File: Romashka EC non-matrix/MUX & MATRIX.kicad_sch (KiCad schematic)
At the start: 65 parts, among them SW1 EC_SW, SW10 EC_SW, SW11 EC_SW, SW12 EC_SW, SW13 EC_SW, SW14 EC_SW, SW15 EC_SW, SW16 EC_SW, SW17 EC_SW, SW18 EC_SW, SW19 EC_SW, SW2 EC_SW, SW20 EC_SW, SW21 EC_SW, SW22 EC_SW, SW23 EC_SW, SW24 EC_SW, SW25 EC_SW, SW26 EC_SW, SW27 EC_SW, SW28 EC_SW, SW29 EC_SW, SW3 EC_SW, SW30 EC_SW, SW31 EC_SW, SW32 EC_SW, SW33 EC_SW, SW34 EC_SW, SW35 EC_SW, SW36 EC_SW, SW37 EC_SW, SW38 EC_SW, SW39 EC_SW, SW4 EC_SW, SW40 EC_SW, SW41 EC_SW, SW42 EC_SW, SW43 EC_SW, SW44 EC_SW, SW45 EC_SW, SW46 EC_SW, SW47 EC_SW, SW48 EC_SW, SW49 EC_SW, SW5 EC_SW, SW6 EC_SW, SW7 EC_SW, SW8 EC_SW, SW9 EC_SW, U4 TMUX1308, U5 TMUX1308, U6 TMUX1308, U7 TMUX1308, U8 TMUX1308, U9 TMUX1308

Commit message: 21.04.2026 09:06
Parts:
- removed U4, U5, U6, U7, U8, U9: TMUX1308, Package_SO:TSSOP-16_4.4x5mm_P0.65mm, symbol Analog_Switch:TMUX1208PW
- added C26, C30, C33: 100nF, Capacitor_SMD:C_0402_1005Metric, symbol Device:C_Small
- added C27, C28, C29, C31, C32, C34: 50-100pF, Capacitor_SMD:C_0603_1608Metric, symbol Device:C_Small
- added R13, R17, R20, R23, R26, R29: 33K, Resistor_SMD:R_0603_1608Metric, symbol Device:R_Small
- added R14, R15, R16, R18, R19, R21, R22, R24, R25, R27, R28, R30: 330R, Resistor_SMD:R_0603_1608Metric, symbol Device:R_Small
- added U10, U11, U12: OPA2365, Package_SO:SOIC-8_3.9x4.9mm_P1.27mm, symbol Amplifier_Operational:OPA2376xxD
- added U4, U5, U6, U7, U8, U9: 4051, Package_SO:TSSOP-16_4.4x5mm_P0.65mm, symbol 4xxx:4051
- SW1, SW13, SW14, SW2, SW3, SW6, SW7: footprint Kicad footprints:ecs_pad_1U_hybrid_hotswap_V3 -> Kicad footprints:ecs_pad_1U_hybrid_hotswap_V3_switched_sides
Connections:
- net +3.3VA: now also C26.2, C30.2, C33.2, U10.8 (V+), U11.8 (V+), U12.8 (V+), U4.16 (VDD), U5.16 (VDD), U6.16 (VDD), U7.16 (VDD), U8.16 (VDD), U9.16 (VDD)
- net COM0: now also C27.1, U10.3 (+), U4.3 (X)
- net COM1: now also C28.1, U10.5 (+), U5.3 (X)
- net COM2: now also C29.1, U11.3 (+), U6.3 (X)
- net COM3: now also C31.1, U11.5 (+), U7.3 (X)
- net COM4: now also C32.1, U12.3 (+), U8.3 (X)
- net COM5: now also C34.1, U12.5 (+), U9.3 (X)
- net DRIVE_MUX0: now also SW13.2, SW14.2; no longer SW7.2, SW8.2
- net DRIVE_MUX1: now also SW20.2, SW21.2, SW22.2, SW23.2; no longer SW13.2, SW14.2
- net DRIVE_MUX2: no longer SW20.2, SW21.2, SW22.2, SW23.2
- net EC_SW1: now also U4.14 (X1)
- net EC_SW10: now also U5.14 (X1)
- net EC_SW11: now also U5.15 (X2)
- net EC_SW12: now also U5.12 (X3)
- net EC_SW13: now also U4.13 (X0)
- net EC_SW14: now also U4.12 (X3)
- net EC_SW17: now also U6.13 (X0)
- net EC_SW18: now also U6.14 (X1)
- net EC_SW19: now also U6.15 (X2)
- net EC_SW2: now also U4.15 (X2)
- net EC_SW20: now also U5.4 (X7), U6.12 (X3)
- net EC_SW21: now also U5.1 (X4), U6.1 (X4)
- net EC_SW22: now also U5.5 (X5), U6.5 (X5)
- net EC_SW23: now also U5.2 (X6), U6.2 (X6)
- net EC_SW24: now also U6.4 (X7)
- net EC_SW25: now also U7.13 (X0)
- net EC_SW26: now also U7.14 (X1)
- net EC_SW27: now also U7.15 (X2)
- net EC_SW28: now also U7.12 (X3)
- net EC_SW29: now also U7.1 (X4)
- net EC_SW3: now also U4.1 (X4)
- net EC_SW30: now also U7.5 (X5)
- net EC_SW31: now also U7.2 (X6)
- net EC_SW32: now also U7.4 (X7)
- net EC_SW33: now also U8.13 (X0)
- net EC_SW34: now also U8.14 (X1)
- net EC_SW35: now also U8.15 (X2)
- net EC_SW36: now also U8.12 (X3)
- net EC_SW37: now also U8.1 (X4)
- net EC_SW38: now also U8.5 (X5)
- net EC_SW39: now also U8.2 (X6)
- net EC_SW4: now also U4.2 (X6)
- net EC_SW40: now also U8.4 (X7)
- net EC_SW41: now also U9.13 (X0)
- net EC_SW42: now also U9.14 (X1)
- net EC_SW43: now also U9.15 (X2)
- net EC_SW44: now also U9.12 (X3)
- net EC_SW45: now also U9.1 (X4)
- net EC_SW46: now also U9.5 (X5)
- net EC_SW47: now also U9.2 (X6)
- net EC_SW5: now also U4.4 (X7)
- net EC_SW6: now also U4.5 (X5)
- net EC_SW9: now also U5.13 (X0)
- net GND: now also C26.1, C27.2, C28.2, C29.2, C30.1, C31.2, C32.2, C33.1, C34.2, R14.2, R18.2, R21.2, R24.2, R27.2, R30.2, U10.4 (V-), U11.4 (V-), U12.4 (V-), U4.6 (Inh), U4.7 (VEE), U4.8 (VSS), U5.6 (Inh), U5.7 (VEE), U5.8 (VSS), U6.6 (Inh), U6.7 (VEE), U6.8 (VSS), U7.6 (Inh), U7.7 (VEE), U7.8 (VSS), U8.6 (Inh), U8.7 (VEE), U8.8 (VSS), U9.6 (Inh), U9.7 (VEE), U9.8 (VSS)
- net MUX_S0: now also U4.11 (A), U5.11 (A), U6.11 (A), U7.11 (A), U8.11 (A), U9.11 (A)
- net MUX_S1: now also U4.10 (B), U5.10 (B), U6.10 (B), U7.10 (B), U8.10 (B), U9.10 (B)
- net MUX_S2: now also U4.9 (C), U5.9 (C), U6.9 (C), U7.9 (C), U8.9 (C), U9.9 (C)
- new net: R22.1, R23.1, U11.7
- new net: R25.1, R26.1, U12.1
- new net: R16.1, R17.1, U10.7
- new net: R17.2, R18.1, U10.6 (-)
- new net: R19.1, R20.1, U11.1
- new net: R20.2, R21.1, U11.2 (-)
- new net: R29.2, R30.1, U12.6 (-)
- new net: R26.2, R27.1, U12.2 (-)
- new net: R13.1, R15.1, U10.1
- new net: R23.2, R24.1, U11.6 (-)
- new net: R28.1, R29.1, U12.7
- new net: R13.2, R14.1, U10.2 (-)
- new net ADC0: R15.2
- new net ADC1: R16.2
- new net ADC2: R19.2
- new net ADC3: R22.2
- new net ADC4: R25.2
- new net ADC5: R28.2
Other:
- moved on the sheet: C20, C21, C22, C23, C24, C25, S38, S39, S46, S49, SW1, SW10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

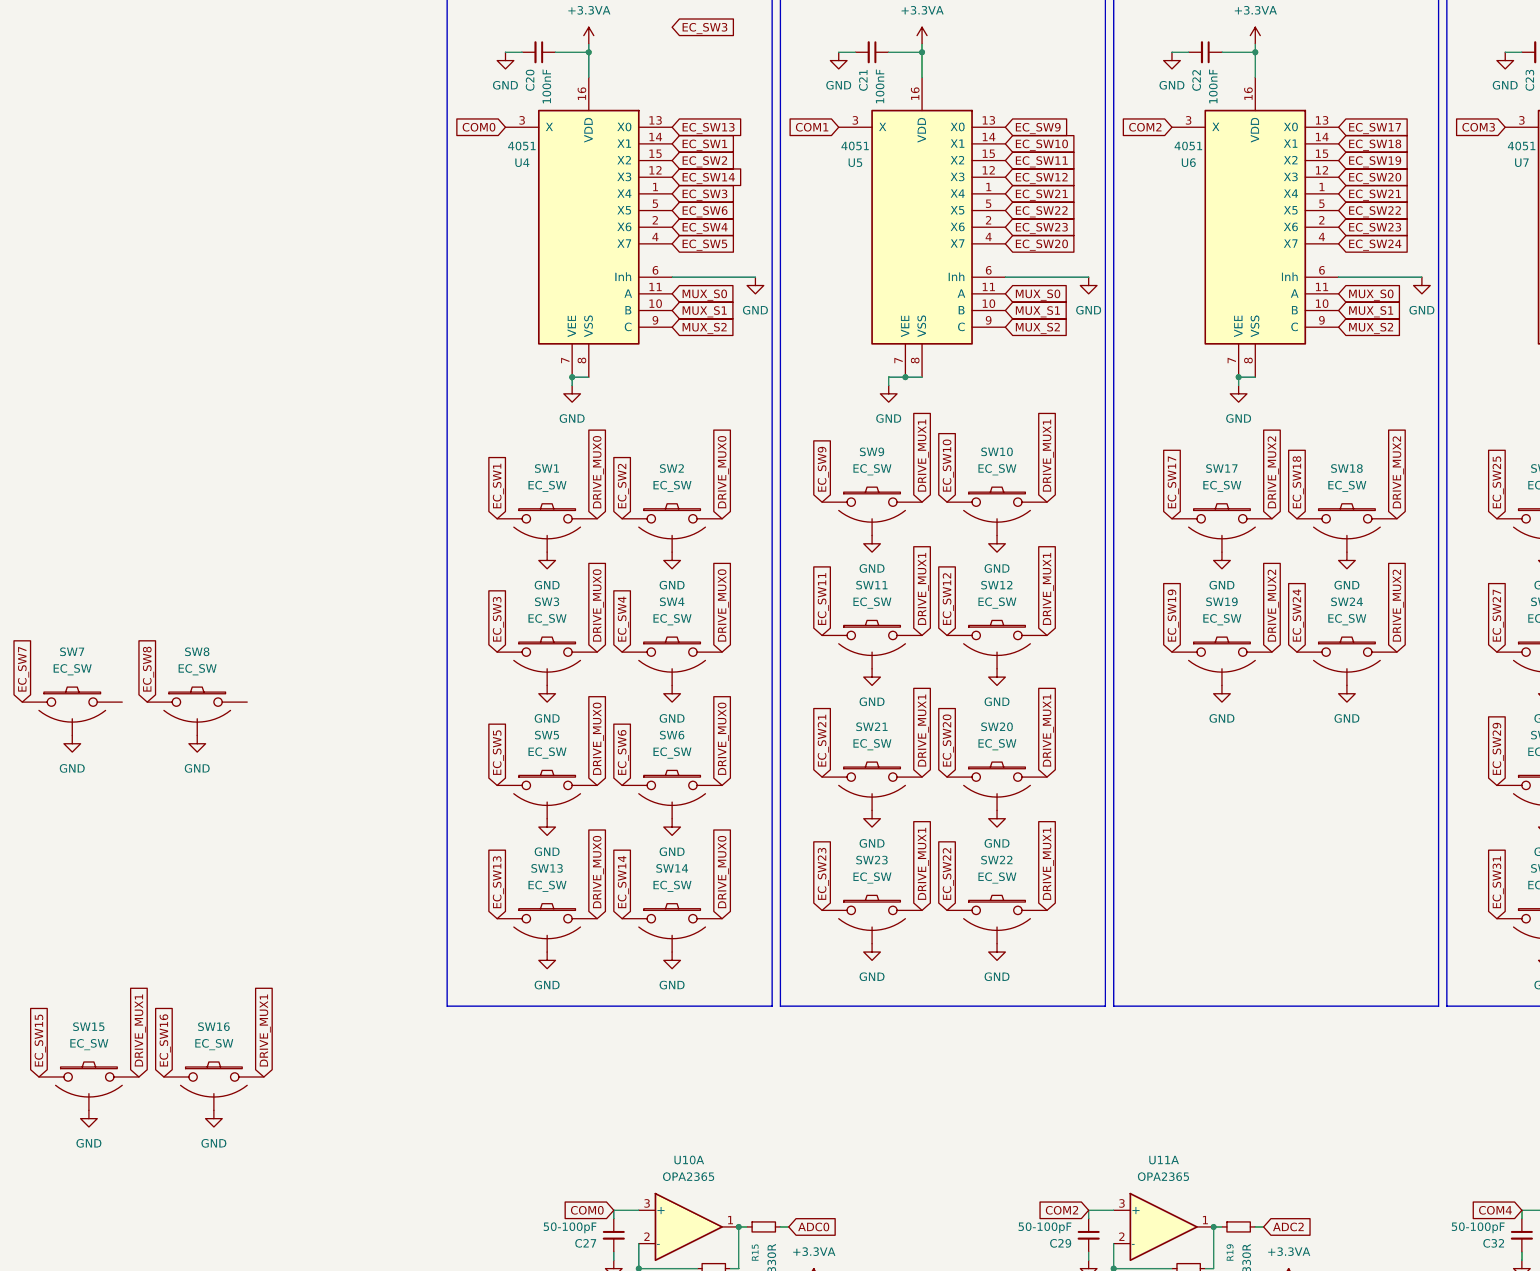
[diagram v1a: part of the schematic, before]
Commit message: 21.04.2026 something something
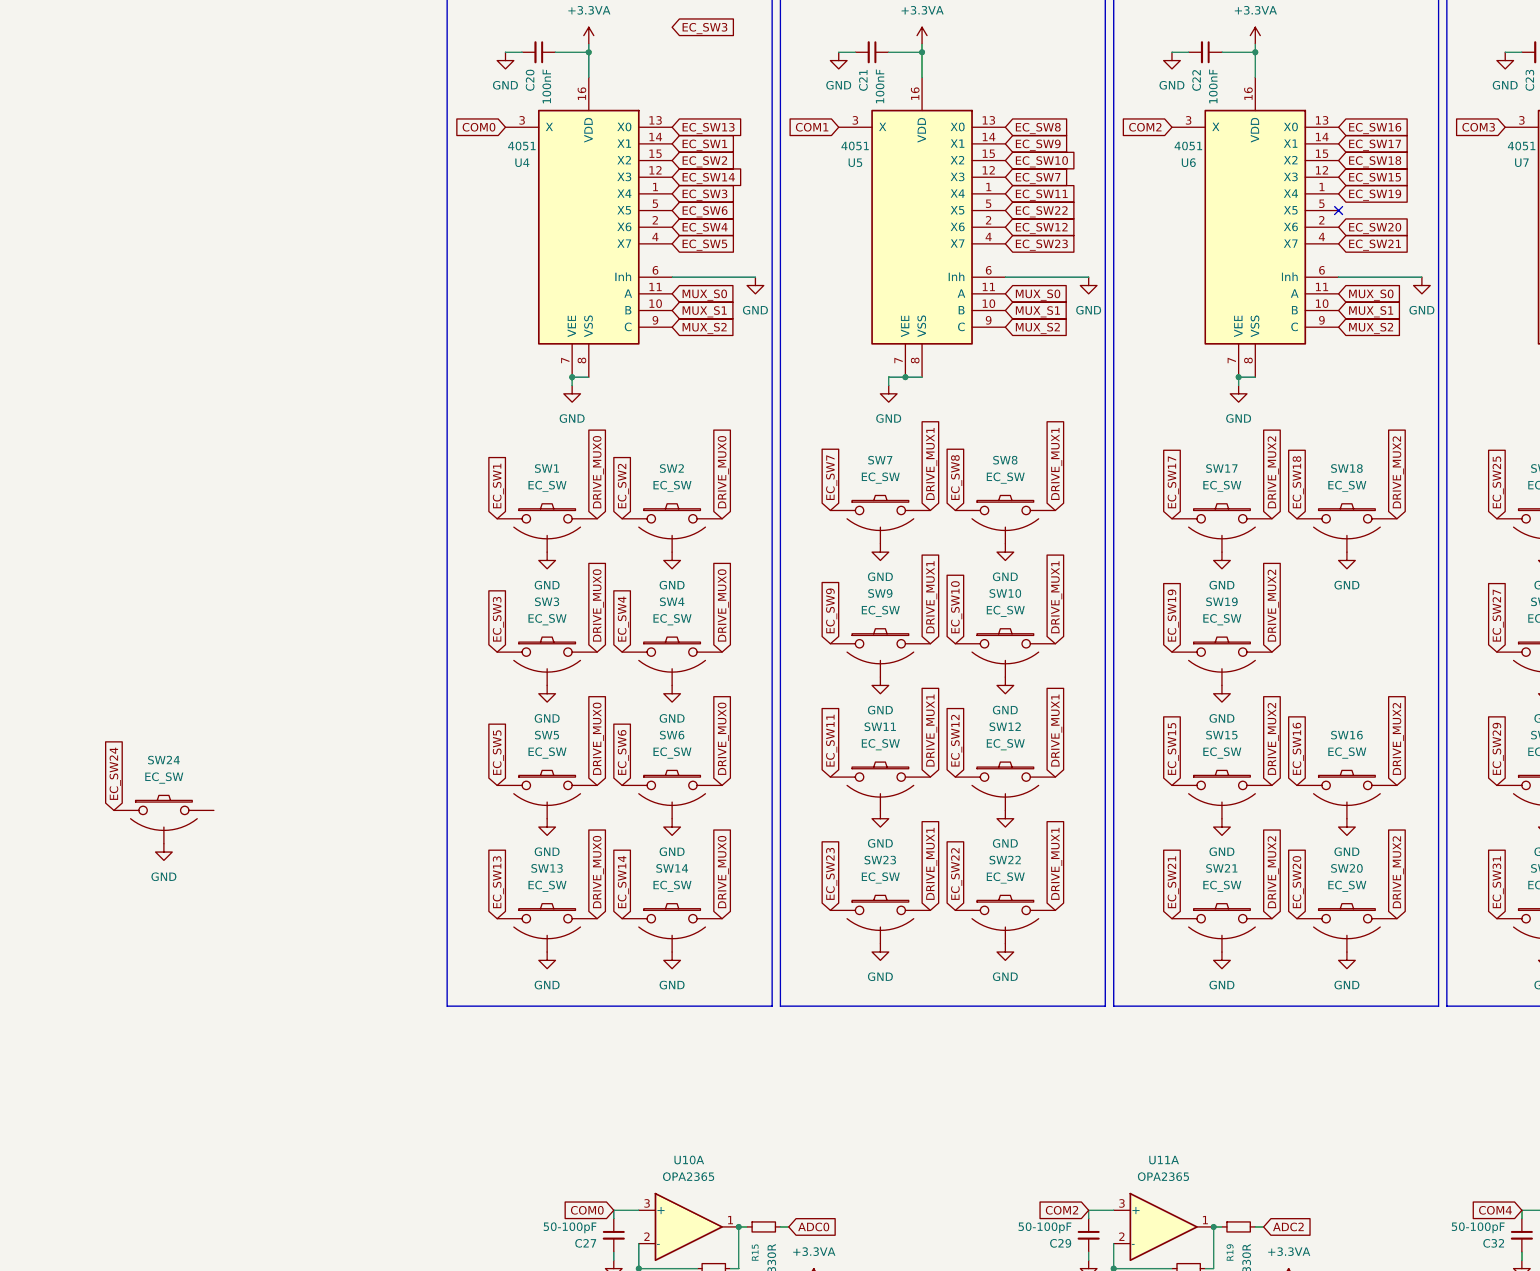
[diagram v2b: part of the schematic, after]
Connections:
- net DRIVE_MUX1: now also SW7.2, SW8.2; no longer SW15.2, SW16.2, SW20.2, SW21.2
- net DRIVE_MUX2: now also SW15.2, SW16.2, SW20.2, SW21.2; no longer SW24.2
- net EC_SW10: now also U5.15 (X2); no longer U5.14 (X1)
- net EC_SW11: now also U5.1 (X4); no longer U5.15 (X2)
- net EC_SW12: now also U5.2 (X6); no longer U5.12 (X3)
- net EC_SW15: now also U6.12 (X3)
- net EC_SW16: now also U6.13 (X0)
- net EC_SW17: now also U6.14 (X1); no longer U6.13 (X0)
- net EC_SW18: now also U6.15 (X2); no longer U6.14 (X1)
- net EC_SW19: now also U6.1 (X4); no longer U6.15 (X2)
- net EC_SW20: now also U6.2 (X6); no longer U5.4 (X7), U6.12 (X3)
- net EC_SW21: now also U6.4 (X7); no longer U5.1 (X4), U6.1 (X4)
- net EC_SW22: no longer U6.5 (X5)
- net EC_SW23: now also U5.4 (X7); no longer U5.2 (X6), U6.2 (X6)
- net EC_SW24: no longer U6.4 (X7)
- net EC_SW7: now also U5.12 (X3)
- net EC_SW8: now also U5.13 (X0)
- net EC_SW9: now also U5.14 (X1); no longer U5.13 (X0)
- no-connect marks 0 -> 1
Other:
- moved on the sheet: SW10, SW11, SW12, SW15, SW16, SW20, SW21, SW22, SW23, SW24, SW7, SW8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
